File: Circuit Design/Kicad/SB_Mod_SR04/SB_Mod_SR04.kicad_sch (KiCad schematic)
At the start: 24 parts, among them J1 TPs, J2 GND, J3 RESET, U1 ATTINY84A

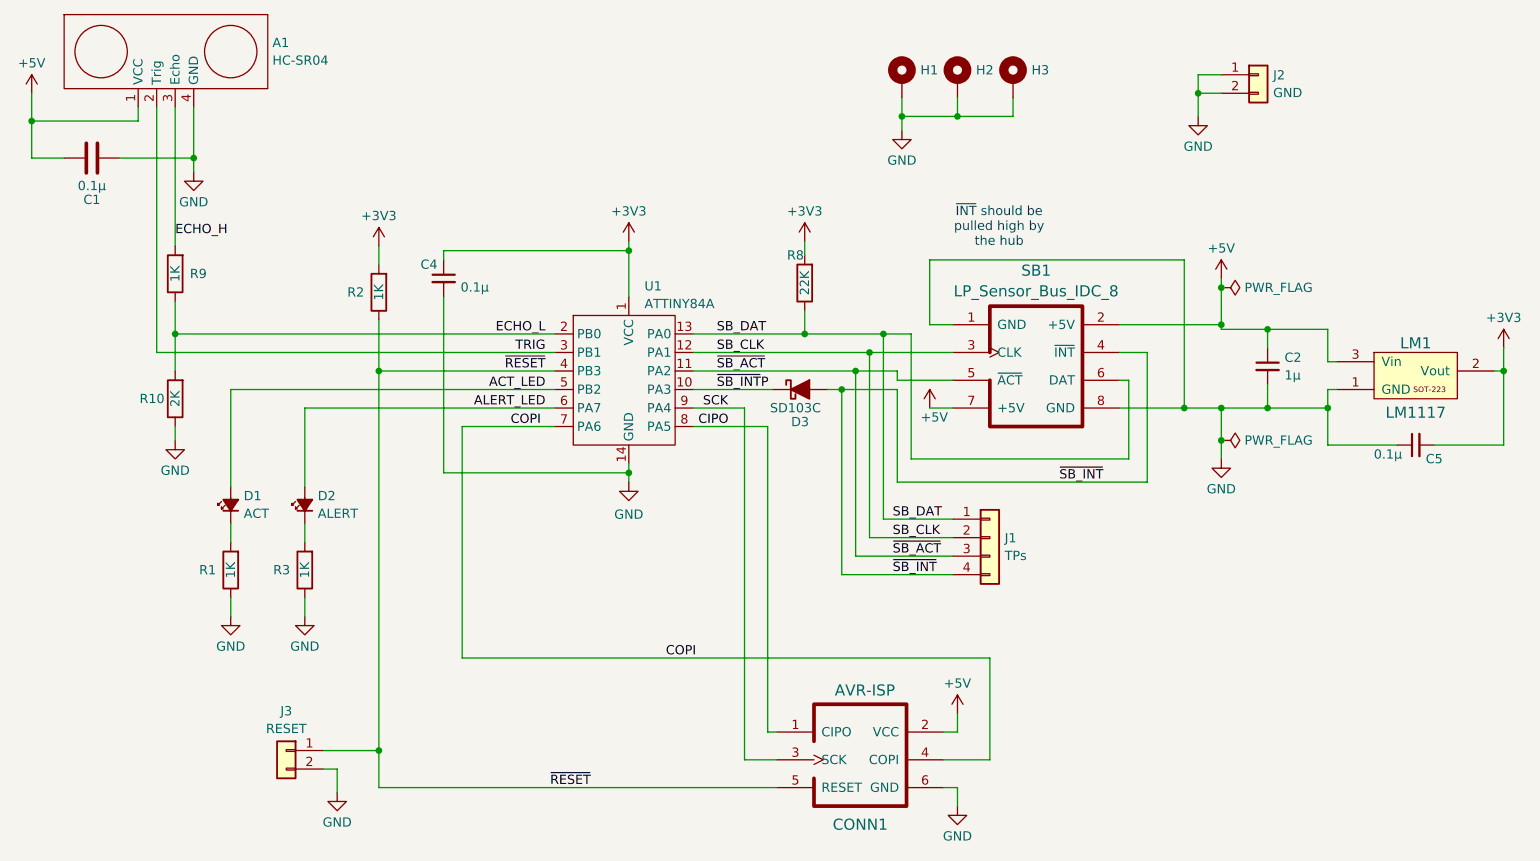
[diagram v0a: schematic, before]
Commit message: Tidy up
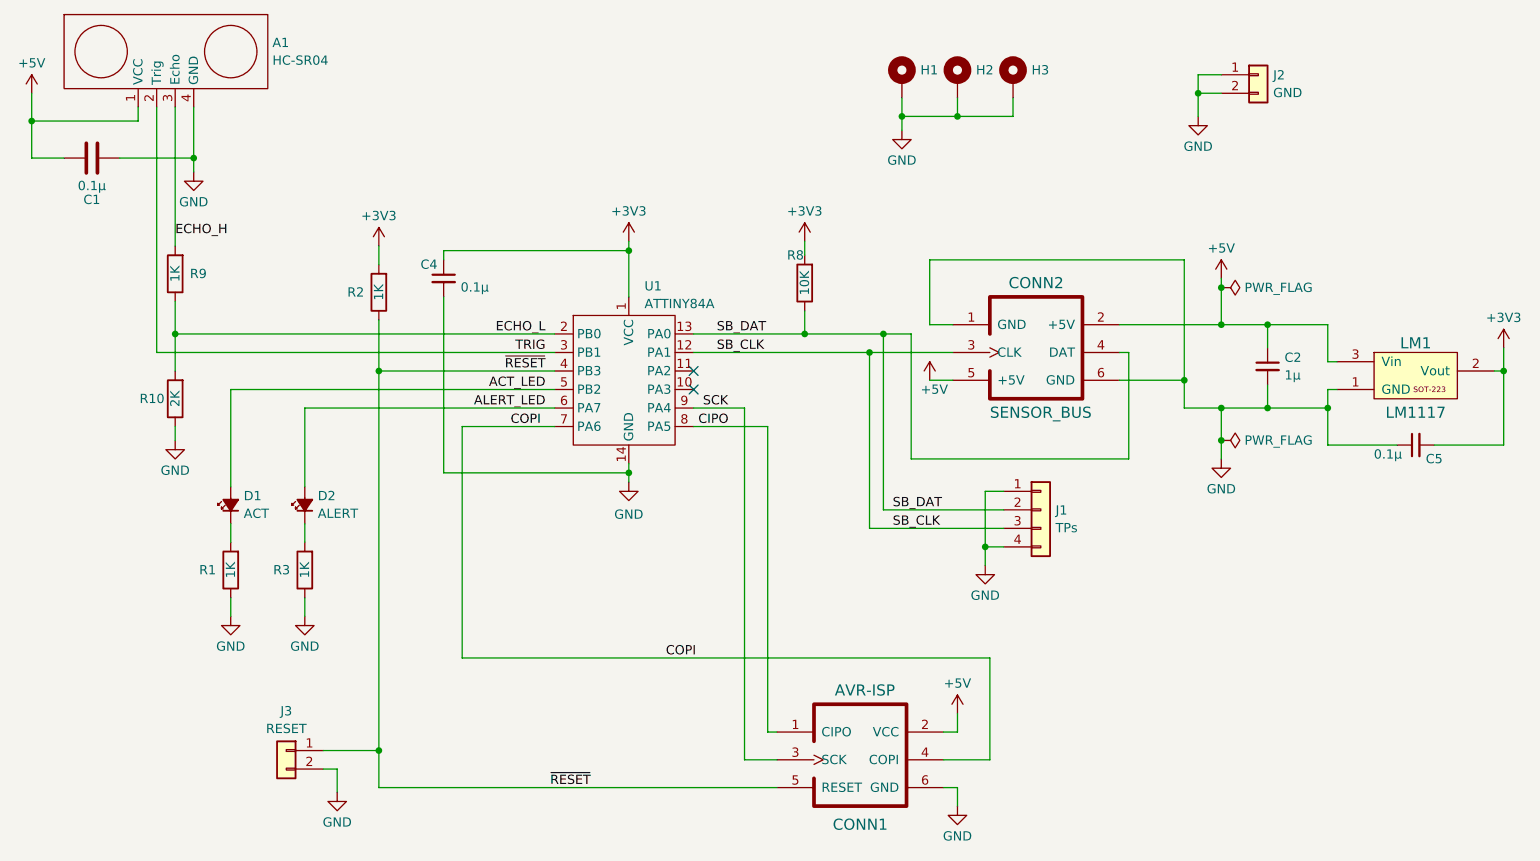
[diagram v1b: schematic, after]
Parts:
- removed D3: SD103C, Diode_SMD:D_SOD-123, symbol Device:D_Schottky_Filled
- removed SB1: LP_Sensor_Bus_IDC_8, MS_Connectors:SensorBus_2x04_P2.54mm_Vertical, symbol MS_Conn:LP_Sensor_Bus_IDC_8
- added CONN2: SENSOR_BUS, MS_Connectors:LP_Sensor_Bus_HE10_2x3, symbol MS_Conn:LP_Sensor_Bus_IDC_6
- C1, C2, C4, C5: Type (none) -> SMD
- R8: value 22K -> 10K
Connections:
- net ~{SB_INT} is gone; now on net GND: J1.4 (Pin_4)
- net +5V: now also CONN2.2 (+5V), CONN2.5 (+5V)
- net GND: now also J1.1 (Pin_1), CONN2.1 (GND), CONN2.6 (GND)
- net SB_CLK: now also J1.3 (Pin_3), CONN2.3 (CLK); no longer J1.2 (Pin_2)
- net SB_DAT: now also J1.2 (Pin_2), CONN2.4 (DAT); no longer J1.1 (Pin_1)
- net ~{SB_ACT}: no longer names the net of U1.11 (PA2)
- net ~{SB_ACT}: no longer J1.3 (Pin_3)
- net ~{SB_INT}P: no longer names the net of U1.10 (PA3)
- no-connect marks 0 -> 2
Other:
- note removed: "~{INT} should be pulled high by the hub"
- moved on the sheet: J1
